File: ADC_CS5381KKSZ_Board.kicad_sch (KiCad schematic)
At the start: 3 parts

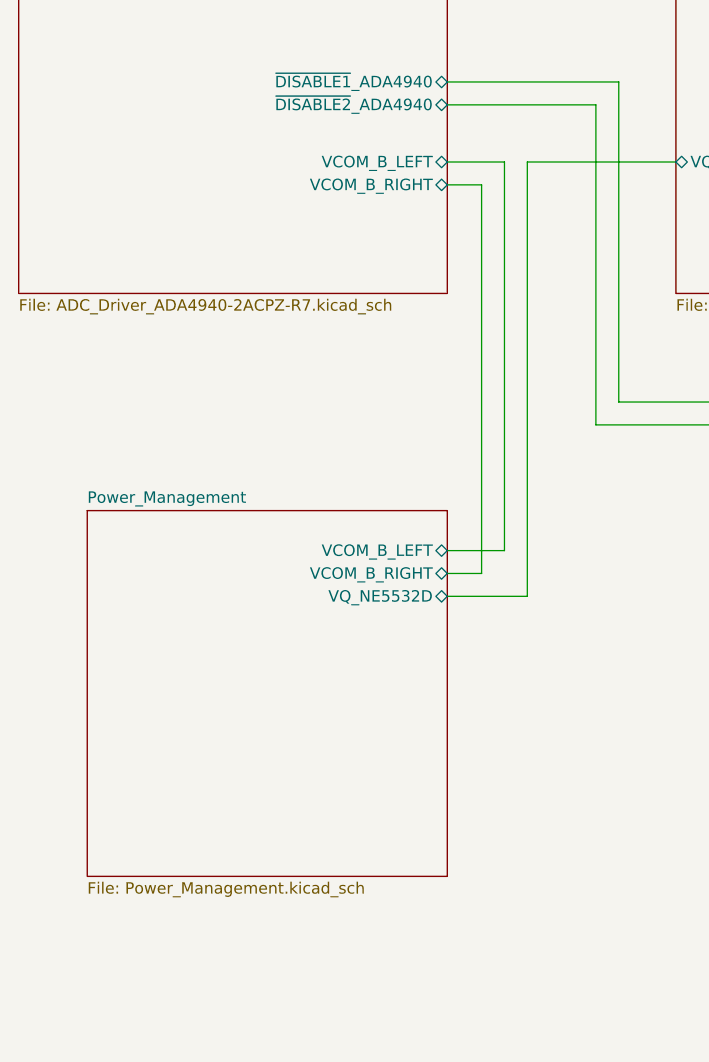
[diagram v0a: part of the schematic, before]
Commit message: Update
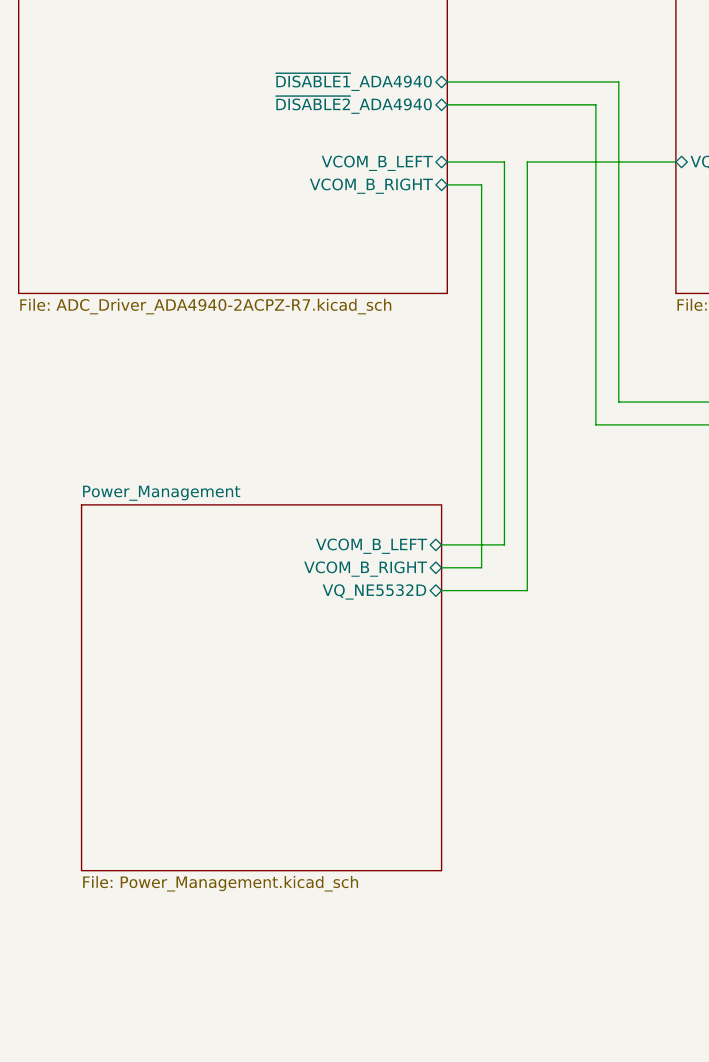
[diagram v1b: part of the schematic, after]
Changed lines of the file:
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@@
 	(wire
 		(pts
-			(xy 93.98 130.81) (xy 90.17 130.81)
+			(xy 93.98 130.175) (xy 89.535 130.175)
 		)
 		(stroke
@@
 	(wire
 		(pts
-			(xy 96.52 128.27) (xy 90.17 128.27)
-		)
-		(stroke
-			(width 0)
-			(type default)
-		)
-	)
-	(wire
-		(pts
-			(xy 93.98 87.63) (xy 93.98 130.81)
+			(xy 96.52 127.635) (xy 89.535 127.635)
+		)
+		(stroke
+			(width 0)
+			(type default)
+		)
+	)
+	(wire
+		(pts
+			(xy 93.98 87.63) (xy 93.98 130.175)
 		)
 		(stroke
@@
 	(wire
 		(pts
-			(xy 99.06 85.09) (xy 99.06 133.35)
+			(xy 99.06 85.09) (xy 99.06 132.715)
 		)
 		(stroke
@@
 	(wire
 		(pts
-			(xy 96.52 85.09) (xy 96.52 128.27)
-		)
-		(stroke
-			(width 0)
-			(type default)
-		)
-	)
-	(wire
-		(pts
-			(xy 99.06 133.35) (xy 90.17 133.35)
+			(xy 96.52 85.09) (xy 96.52 127.635)
+		)
+		(stroke
+			(width 0)
+			(type default)
+		)
+	)
+	(wire
+		(pts
+			(xy 99.06 132.715) (xy 89.535 132.715)
 		)
 		(stroke
@@
 	)
 	(sheet
-		(at 50.165 123.825)
+		(at 49.53 123.19)
 		(size 40.005 40.64)
 		(fields_autoplaced yes)
@@
 		)
 		(property "Sheetname" "Power_Management"
-			(at 50.165 123.1134 0)
+			(at 49.53 122.4784 0)
 			(effects
 				(font
@@
 		)
 		(property "Sheetfile" "Power_Management.kicad_sch"
-			(at 50.165 165.0496 0)
+			(at 49.53 164.4146 0)
 			(effects
 				(font
@@
 		)
 		(pin "VCOM_B_LEFT" bidirectional
-			(at 90.17 128.27 0)
+			(at 89.535 127.635 0)
 			(effects
 				(font
@@
 		)
 		(pin "VQ_NE5532D" bidirectional
-			(at 90.17 133.35 0)
+			(at 89.535 132.715 0)
 			(effects
 				(font
@@
 		)
 		(pin "VCOM_B_RIGHT" bidirectional
-			(at 90.17 130.81 0)
-			(effects
-				(font
+			(at 89.535 130.175 0)
+			(effects
+				(font
